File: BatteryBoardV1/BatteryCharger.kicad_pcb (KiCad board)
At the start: 2 copper layers, 49.5 x 50.8 mm, 12 parts, among them U1 MCP73213

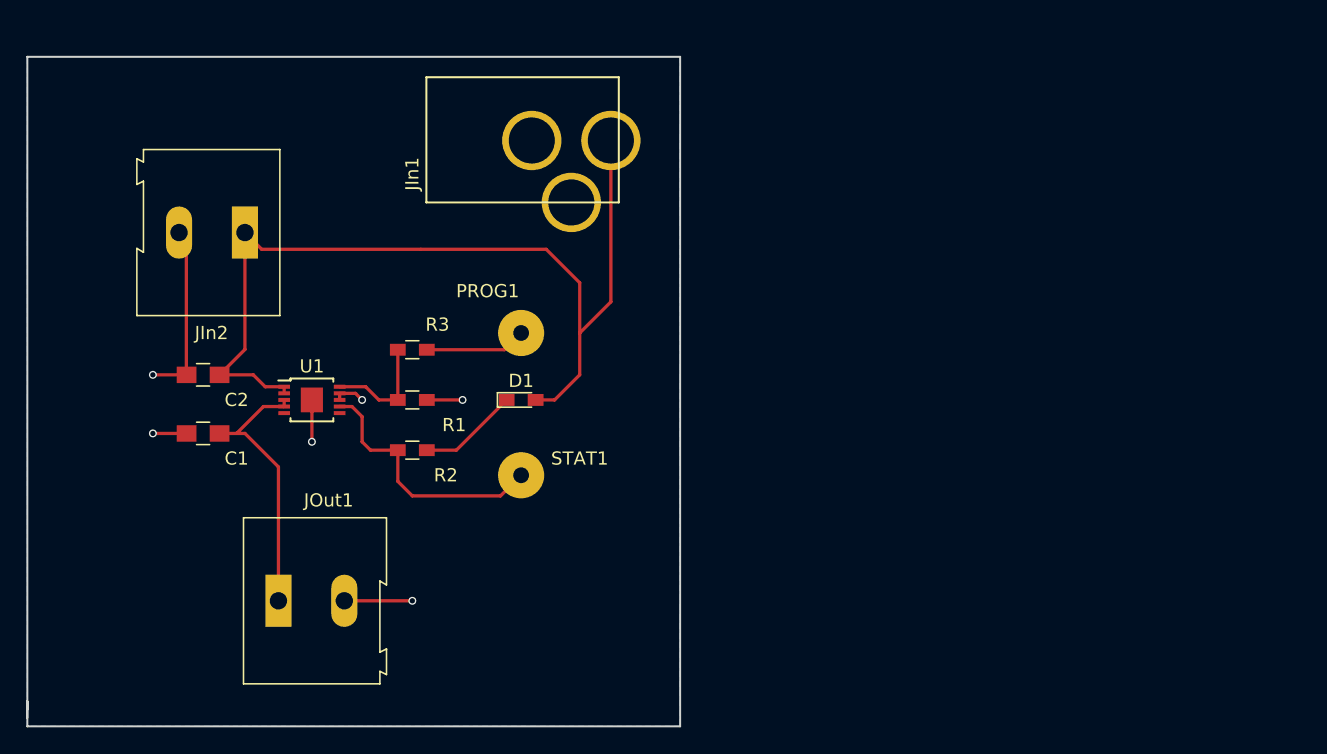
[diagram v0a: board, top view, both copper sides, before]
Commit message: Add files via upload
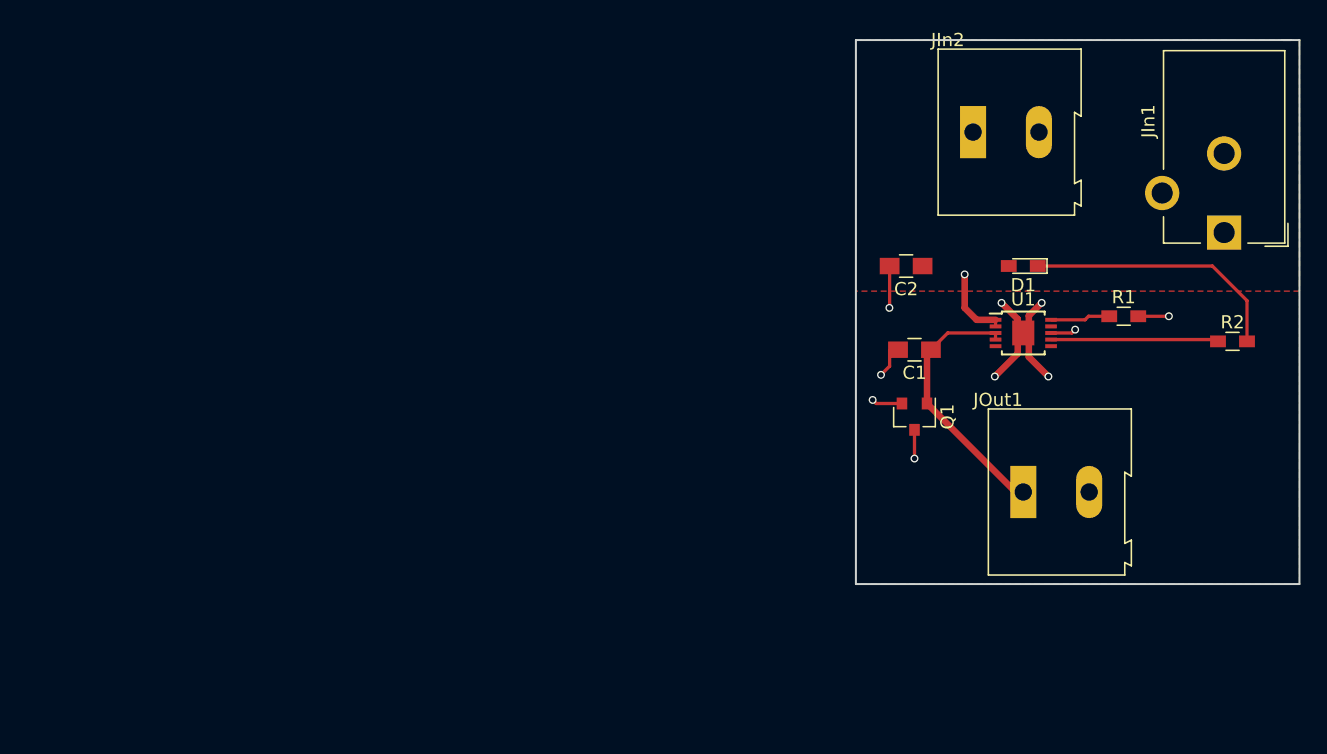
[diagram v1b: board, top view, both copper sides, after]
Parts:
- removed PROG1: TP5, Wire_Pads:SolderWirePad_single_1-2mmDrill
- removed R3: 2.37K, Resistors_SMD:R_0603_HandSoldering
- removed STAT1: TP6, Wire_Pads:SolderWirePad_single_1-2mmDrill
- added Q1: Q_NMOS_GSD, TO_SOT_Packages_SMD:SOT-23, F.Cu at (142.2, 104.1)
- JIn1: footprint BJCs:DC_2.1mm_CUI-PJ-202A -> Connectors:Barrel_Jack_CUI_PJ-102AH
- R1: value 2.37K -> 1.185K
- moved R2 62.8 mm to (166.4, 98.4)
- moved JOut1 57.1 mm to (150.5, 109.9)
- moved JIn2 55.8 mm to (146.7, 82.5), turned to 0 degrees
- moved C1 54.3 mm to (142.2, 99.1)
- moved R1 54.3 mm to (158.1, 96.5)
- moved U1 54.2 mm to (150.5, 97.8)
- moved C2 54.0 mm to (141.6, 92.7)
- moved JIn1 50.0 mm to (165.7, 90.2)
- moved D1 39.4 mm to (150.5, 92.7), turned to 180 degrees
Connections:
- U1 pad 9: GND -> Net-(U1-Pad9)
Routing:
- net VDD: track 71.0 -> 5.75 mm, vias 0 -> 1
- net Net-(D1-Pad1): track 7.63 -> 20.1 mm
- net Net-(PROG1-Pad1): track 7.68 -> 0.00 mm
- net GND: track 33.1 -> 25.7 mm, vias 6 -> 10
- net Net-(R2-Pad1): track 19.7 -> 12.7 mm
- net Net-(R1-Pad1): track 8.64 -> 4.53 mm
- added copper zone on F.Cu, net VDD
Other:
- board size 49.5 x 50.8 mm -> 33.7 x 41.3 mm
- net class High Current added: clearance 0.2, trace_width 0.5, via_dia 0.6, via_drill 0.4
- net class Less High Current added: clearance 0.2, trace_width 0.3, via_dia 0.6, via_drill 0.4

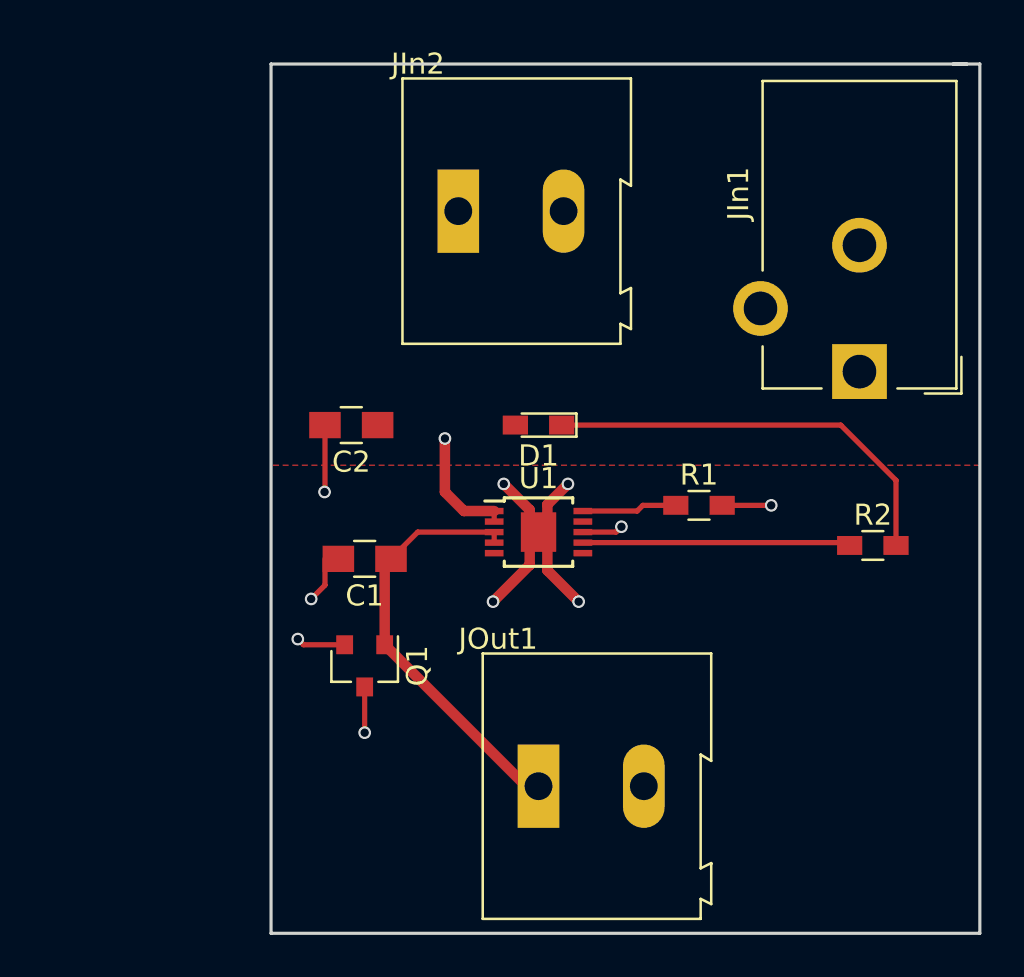
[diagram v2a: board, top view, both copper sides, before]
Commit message: Add files via upload
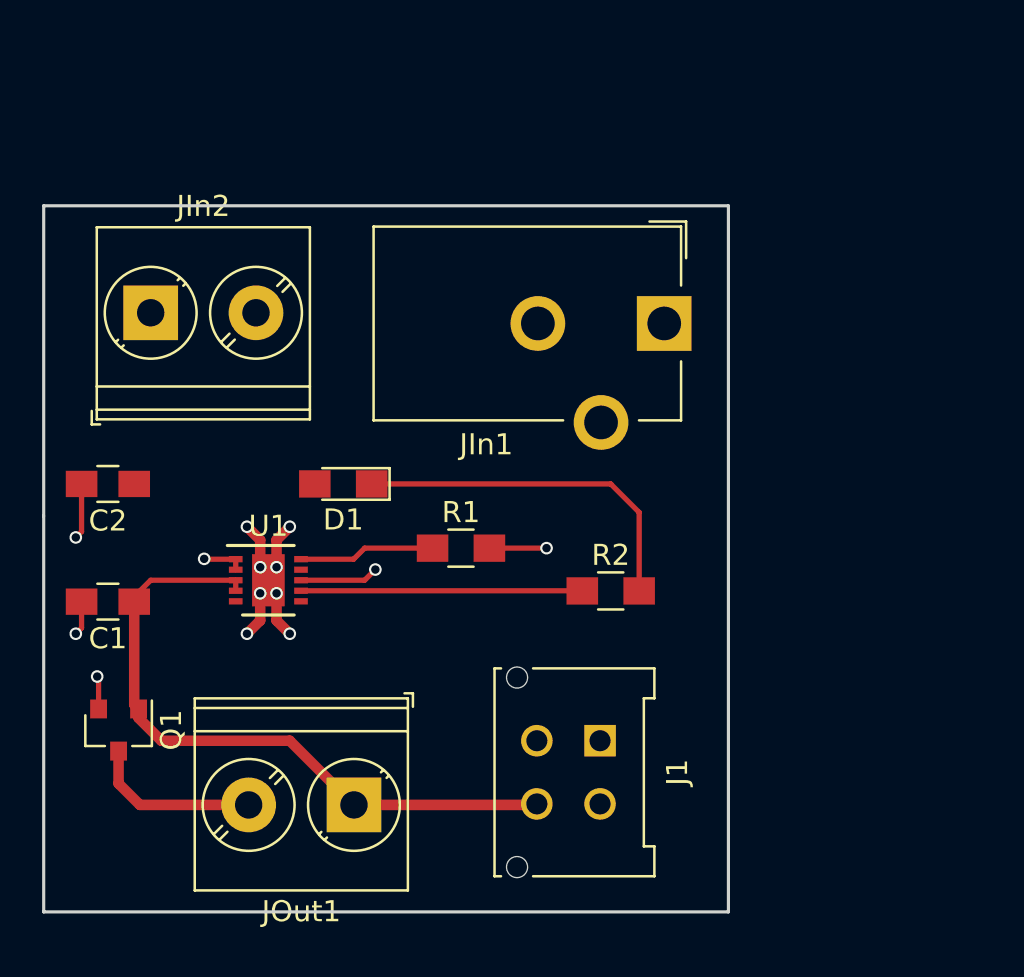
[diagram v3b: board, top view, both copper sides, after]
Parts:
- added J1: Conn_01x04_Male, Connector_Molex:Molex_Micro-Fit_3.0_43045-0412_2x02_P3.00mm_Vertical, F.Cu at (153.4, 107.7)
- D1: footprint LEDs:LED_0603_HandSoldering -> LEDs:LED_0805_HandSoldering
- JIn2, JOut1: footprint Connectors_Terminal_Blocks:TerminalBlock_Altech_AK300-2_P5.00mm -> TerminalBlock_Phoenix:TerminalBlock_Phoenix_PT-1,5-2-5.0-H_1x02_P5.00mm_Horizontal
- R1: value 1.185K -> 3K; footprint Resistors_SMD:R_0603_HandSoldering -> Resistors_SMD:R_0805_HandSoldering
- R2: footprint Resistors_SMD:R_0603_HandSoldering -> Resistors_SMD:R_0805_HandSoldering
- U1: footprint Housings_SSOP:MSOP-10-1EP_3x3mm_Pitch0.5mm -> Housings_DFN_QFN:DFN-10-1EP_3x3mm_Pitch0.5mm
- moved JIn2 15.4 mm to (132.1, 87.4)
- moved U1 13.0 mm to (137.7, 100.1)
- moved R2 12.6 mm to (153.9, 100.6)
- moved C1 12.4 mm to (130.0, 101.1)
- moved Q1 12.1 mm to (130.6, 107.2)
- moved C2 11.9 mm to (130.0, 95.5)
- moved R1 11.5 mm to (146.8, 98.6)
- moved D1 9.68 mm to (141.2, 95.5)
- moved JIn1 9.55 mm to (156.5, 87.9), turned to 270 degrees
- moved JOut1 8.81 mm to (141.7, 110.7), turned to 180 degrees
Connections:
- net Net-(C1-Pad1) renamed /VBAT+
- JOut1 pad 2: GND -> /VBAT-
- Q1 pad 3: GND -> /VBAT-
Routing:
- net /VBAT+: track 20.2 -> 32.1 mm
- net /VBAT-: track 0.00 -> 8.14 mm
- net GND: track 25.7 -> 21.0 mm, vias 10 -> 13
- net VDD: track 5.75 -> 2.00 mm
- net Net-(D1-Pad1): track 20.1 -> 17.0 mm
- net Net-(R1-Pad1): track 4.53 -> 6.46 mm
- net Net-(R2-Pad1): track 12.7 -> 13.4 mm
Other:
- board size 33.7 x 41.3 mm -> 32.5 x 33.5 mm
